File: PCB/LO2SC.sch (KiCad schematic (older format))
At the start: 3 parts, among them P1 CONN_01X05, P2 CONN_01X05, P3 CONN_01X10

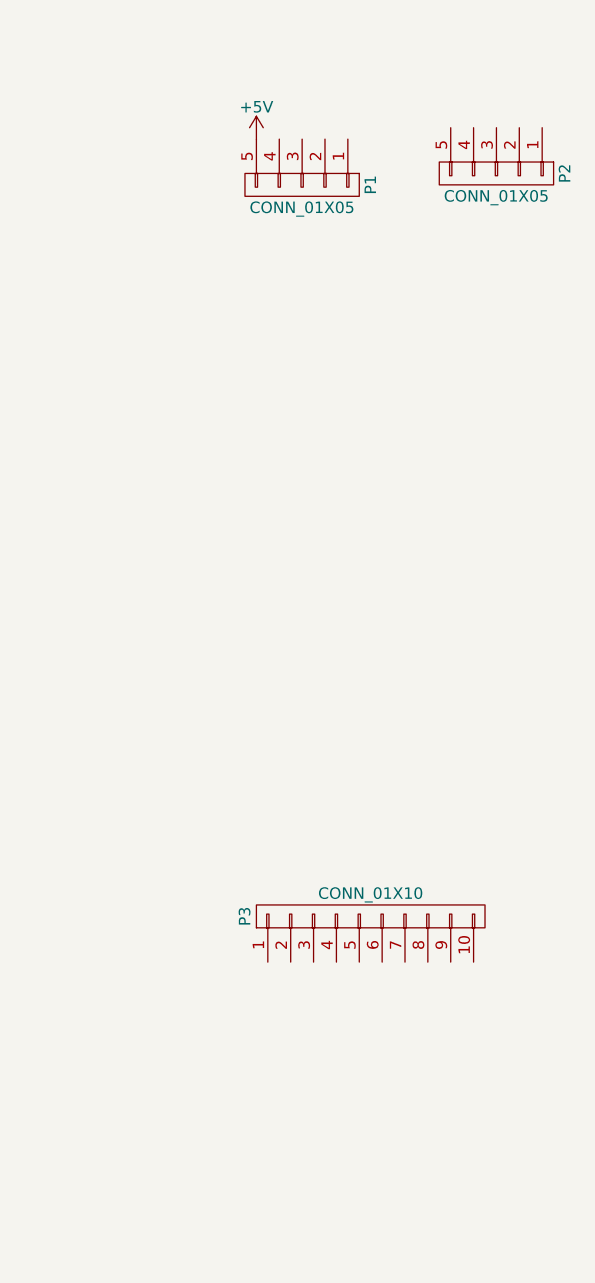
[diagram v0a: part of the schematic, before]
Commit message: ?
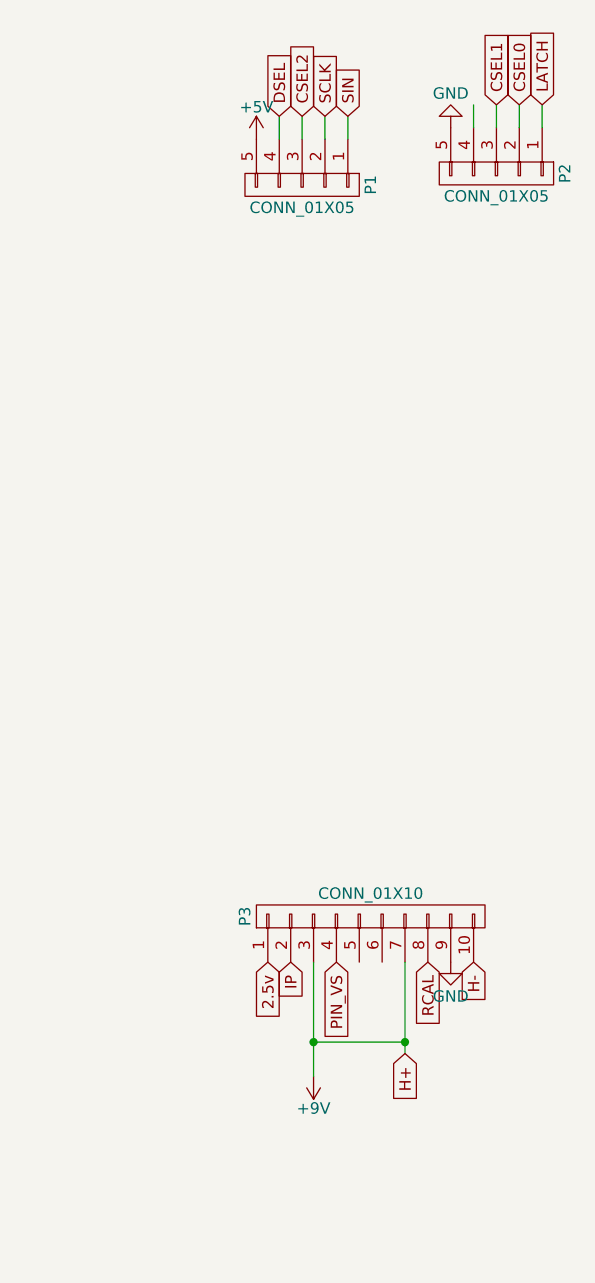
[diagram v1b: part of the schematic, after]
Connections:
- net labels added: +9V, 2.5v, CSEL0, CSEL1, CSEL2, DSEL, GND, H+, H-, IP, LATCH, PIN_VS, RCAL, SCLK, SIN
- wire segments 0 -> 11
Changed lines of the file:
@@
 $EndComp
 $Comp
-L +5V #PWR?
+L +5V #PWR01
 U 1 1 56030C63
 P 5950 1800
-F 0 "#PWR?" H 5950 1650 50  0001 C CNN
+F 0 "#PWR01" H 5950 1650 50  0001 C CNN
 F 1 "+5V" H 5950 1940 50  0000 C CNN
 F 2 "" H 5950 1800 60  0000 C CNN
@@
 	1    0    0    -1
 $EndComp
+Wire Wire Line
+	6050 1800 6050 1700
+Text GLabel 6050 1700 1    50   Input ~ 0
+DSEL
+Wire Wire Line
+	6150 1800 6150 1700
+Wire Wire Line
+	6250 1800 6250 1700
+Wire Wire Line
+	6350 1800 6350 1700
+Text GLabel 6150 1700 1    50   Input ~ 0
+CSEL2
+Text GLabel 6250 1700 1    50   Input ~ 0
+SCLK
+Text GLabel 6350 1700 1    50   Input ~ 0
+SIN
+$Comp
+L GND #PWR02
+U 1 1 5603DF84
+P 6800 1750
+F 0 "#PWR02" H 6800 1500 50  0001 C CNN
+F 1 "GND" H 6800 1600 50  0000 C CNN
+F 2 "" H 6800 1750 60  0000 C CNN
+F 3 "" H 6800 1750 60  0000 C CNN
+	1    6800 1750
+	-1   0    0    1
+$EndComp
+Wire Wire Line
+	6900 1750 6900 1650
+Wire Wire Line
+	7000 1750 7000 1650
+Wire Wire Line
+	7100 1750 7100 1650
+Wire Wire Line
+	7200 1750 7200 1650
+Text GLabel 7100 1650 1    50   Input ~ 0
+CSEL0
+Text GLabel 7000 1650 1    50   Input ~ 0
+CSEL1
+Text GLabel 7200 1650 1    50   Input ~ 0
+LATCH
+Wire Wire Line
+	6200 5400 6200 5900
+$Comp
+L +9V #PWR03
+U 1 1 5603EA59
+P 6200 5900
+F 0 "#PWR03" H 6200 5750 50  0001 C CNN
+F 1 "+9V" H 6200 6040 50  0000 C CNN
+F 2 "" H 6200 5900 60  0000 C CNN
+F 3 "" H 6200 5900 60  0000 C CNN
+	1    6200 5900
+	-1   0    0    1
+$EndComp
+Text GLabel 6300 5400 3    50   Input ~ 0
+PIN_VS
+Text GLabel 6000 5400 3    50   Input ~ 0
+2.5v
+Text GLabel 6100 5400 3    50   Input ~ 0
+IP
+Text GLabel 6700 5400 3    50   Input ~ 0
+RCAL
+Text GLabel 6600 5800 3    50   Input ~ 0
+H+
+Text GLabel 6900 5400 3    50   Input ~ 0
+H-
+$Comp
+L GND #PWR04
+U 1 1 5603F1CE
+P 6800 5400
+F 0 "#PWR04" H 6800 5150 50  0001 C CNN
+F 1 "GND" H 6800 5250 50  0000 C CNN
+F 2 "" H 6800 5400 60  0000 C CNN
+F 3 "" H 6800 5400 60  0000 C CNN
+	1    6800 5400
+	1    0    0    -1
+$EndComp
+Wire Wire Line
+	6600 5400 6600 5800
+Wire Wire Line
+	6200 5750 6600 5750
+Connection ~ 6600 5750
+Connection ~ 6200 5750
 $EndSCHEMATC
